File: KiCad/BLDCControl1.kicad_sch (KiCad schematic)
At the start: 36 parts, among them J2 Conn_Power, J3 Conn BLDC, Q1 IRLZ44N, Q2 IRLZ44N, Q3 IRLZ44N, Q4 IRLZ44N, Q5 IRLZ44N, Q6 IRLZ44N, U1 IR2101, U2 IR2101, U3 IR2101, U4 YAAJ_BlackPill_v2, U5 L7805

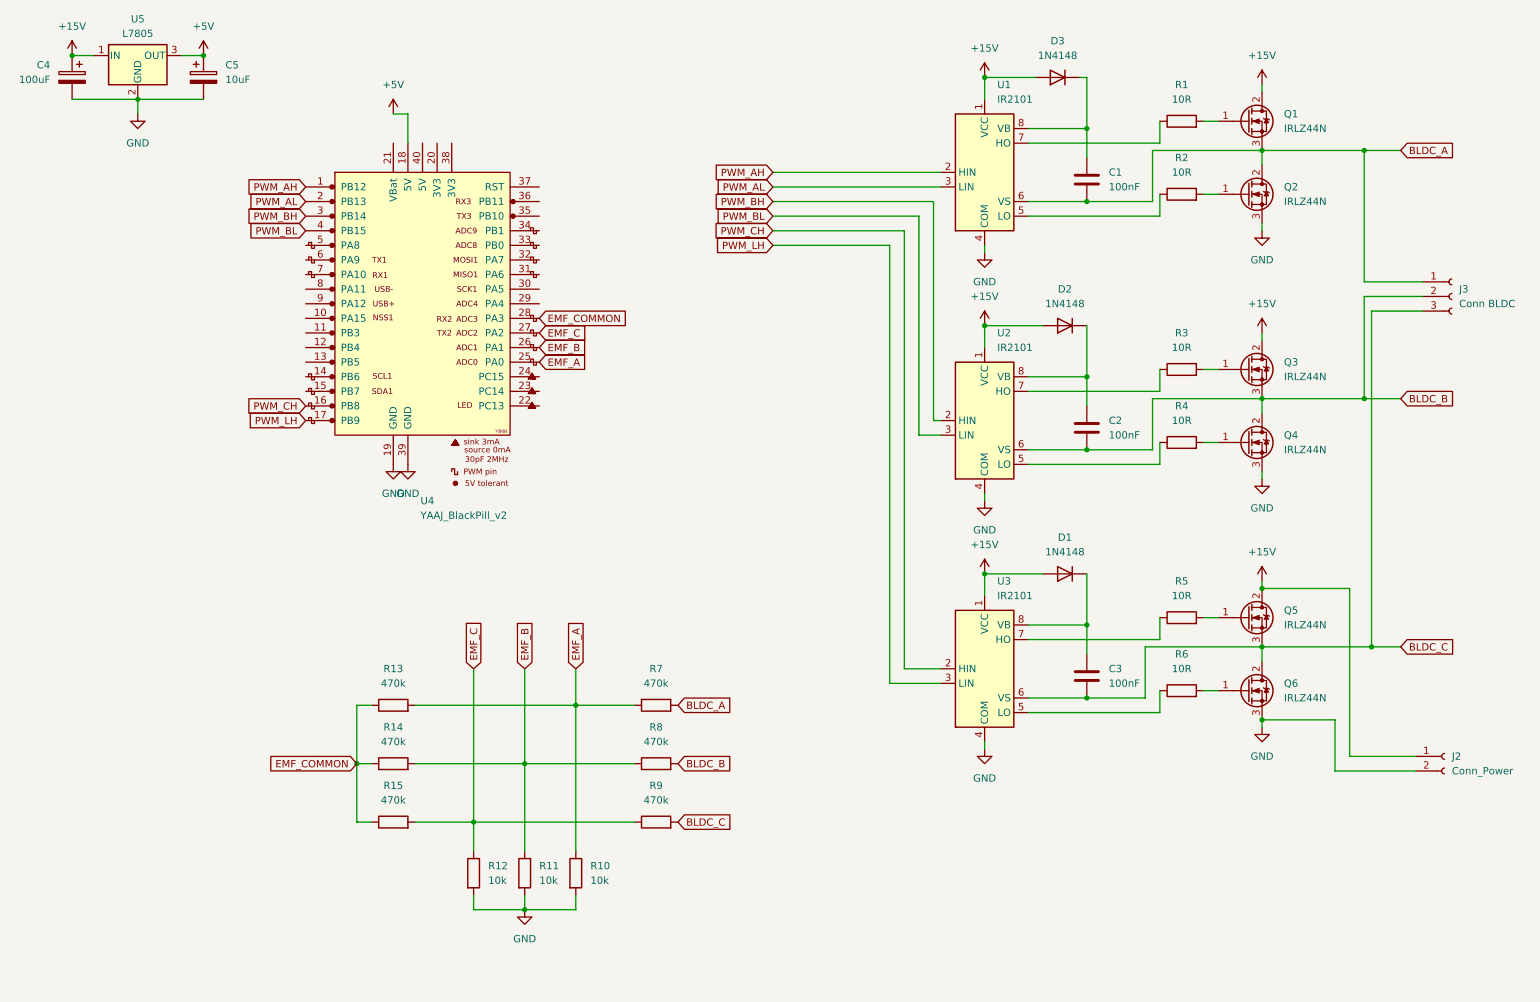
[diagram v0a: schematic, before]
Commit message: KiCad
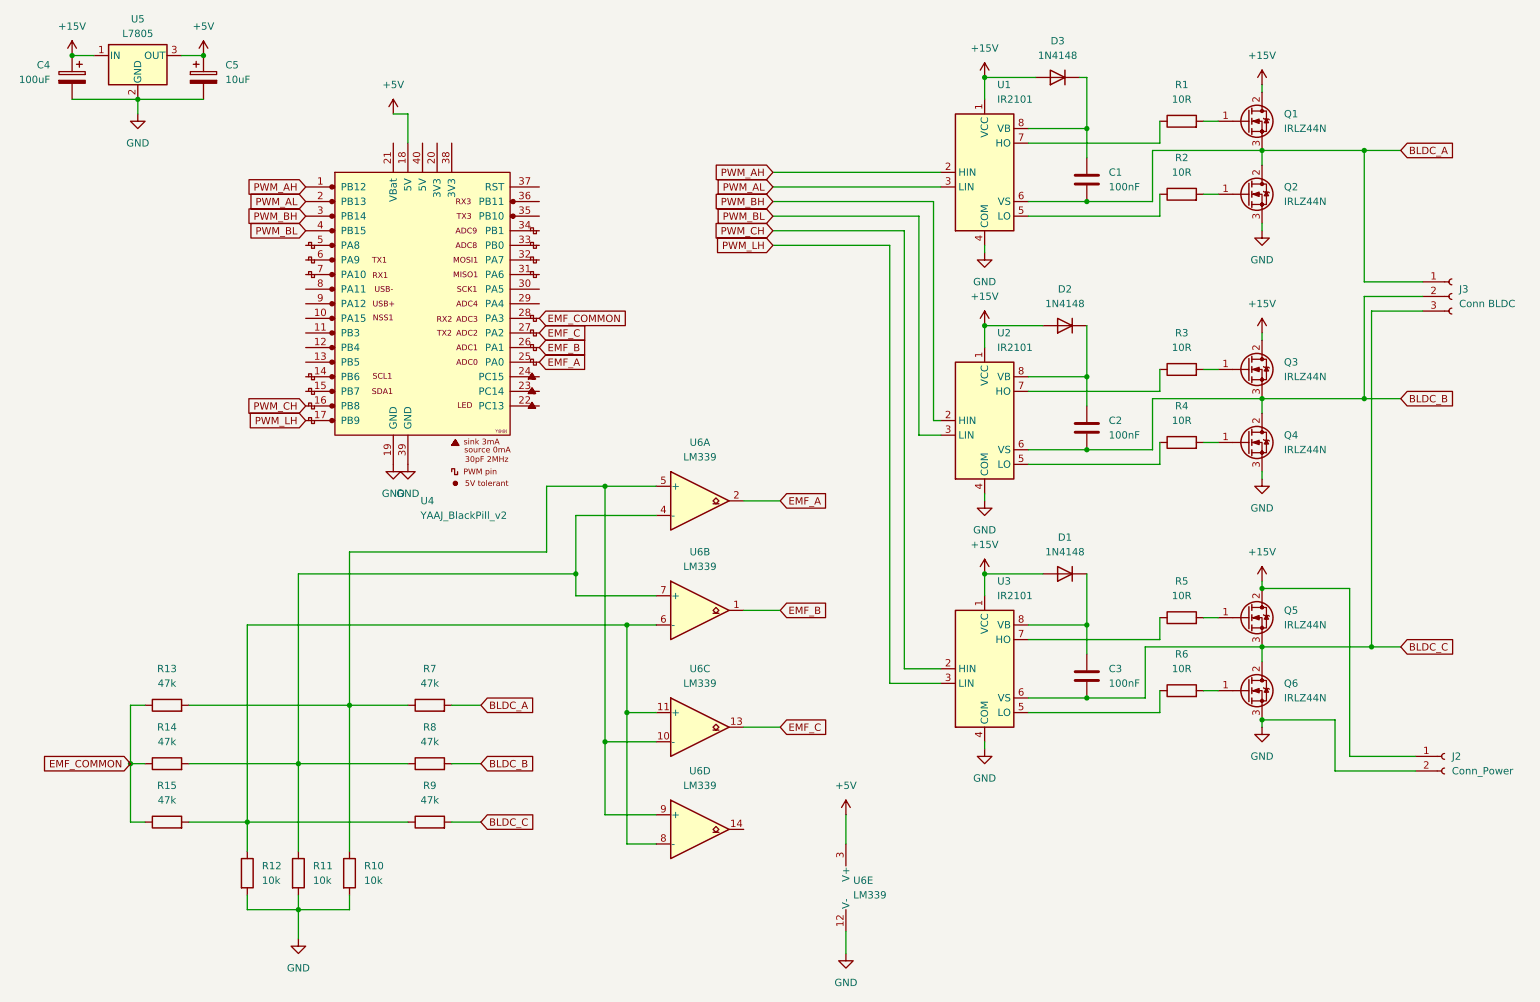
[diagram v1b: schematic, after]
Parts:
- added U6: LM339, symbol Comparator:LM339
- R13, R14, R15, R7, R8, R9: value 470k -> 47k
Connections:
- net +5V: now also U6.3 (V+)
- net EMF_A: now also U6.2; no longer R10.1, R13.2, R7.1
- net EMF_B: now also U6.1; no longer R11.1, R14.2, R8.1
- net EMF_C: now also U6.13; no longer R12.1, R15.2, R9.1
- net GND: now also U6.12 (V-)
- new net: R10.1, R13.2, R7.1, U6.10 (-), U6.5 (+), U6.9 (+)
- new net: R12.1, R15.2, R9.1, U6.11 (+), U6.6 (-), U6.8 (-)
- new net: R11.1, R14.2, R8.1, U6.4 (-), U6.7 (+)
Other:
- moved on the sheet: R10, R11, R12, R13, R14, R15, R7, R8, R9
